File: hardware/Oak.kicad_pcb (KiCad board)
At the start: 2 copper layers, 100 x 40 mm, 73 parts, among them J1 18650 Battery holder, J2 USB_B_Micro, J3 Conn_Coaxial, J4 Conn_ARM_JTAG_SWD_10, SW1 SW_SPDT, SW2 SW_Push, U1 AP2112, U2 ATSAMD21, U3 MCP7383, U4 PA1010D, U5 RFM95, U6 Waveshare_1in54_epaper

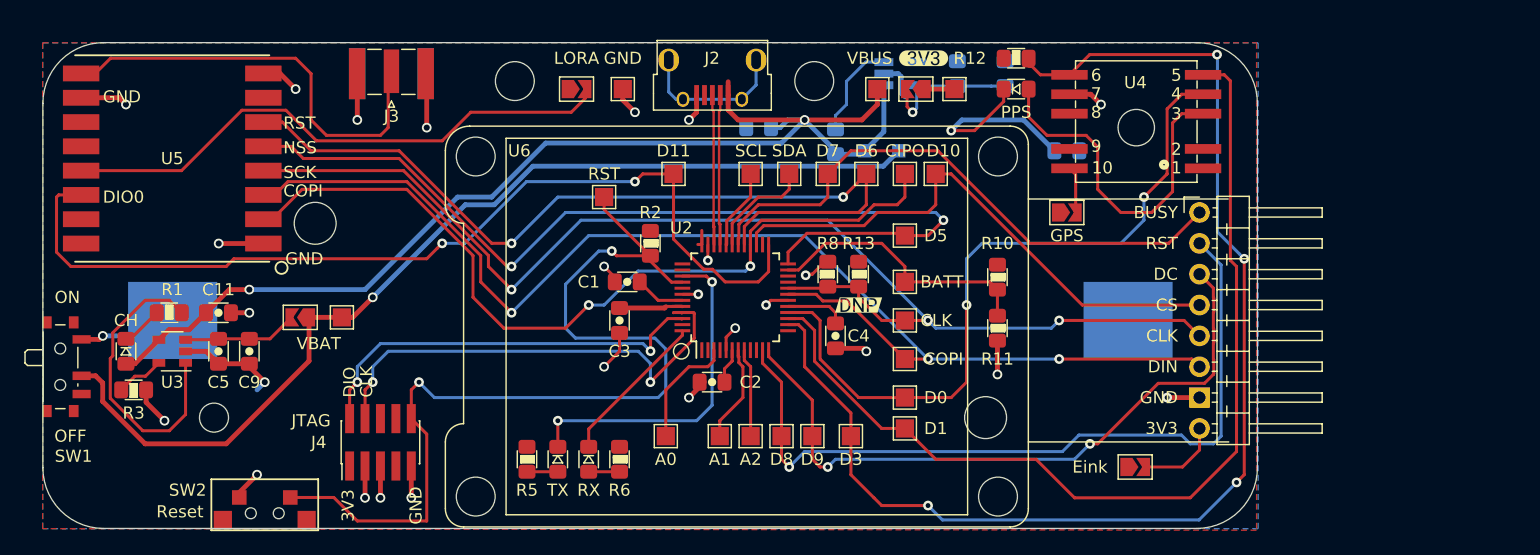
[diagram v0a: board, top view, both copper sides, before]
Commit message: refactor: regenerate drill map files
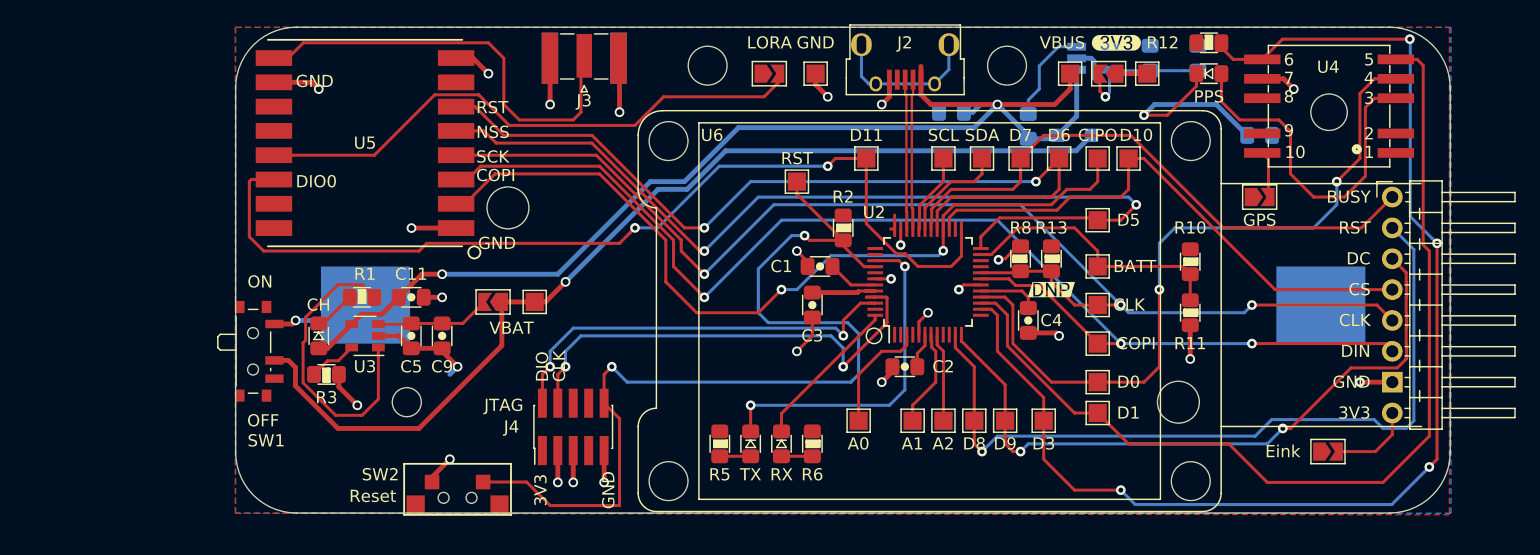
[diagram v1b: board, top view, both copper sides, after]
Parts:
- moved D2 15.9 mm to (45.5, 57.1)
- moved REF** 15.9 mm to (44.5, 66.2)
- moved C1 15.9 mm to (86.7, 51.4)
- moved C10 15.9 mm to (97.5, 38.7)
- moved C11 15.9 mm to (53.1, 54.0)
- moved C2 15.9 mm to (93.7, 59.7)
- moved C3 15.9 mm to (86.1, 54.6)
- moved C4 15.9 mm to (103.9, 55.9)
- moved C5 15.9 mm to (53.1, 57.1)
- moved C6 15.9 mm to (113.9, 34.3)
- moved C7 15.9 mm to (117.8, 34.3)
- moved C9 15.9 mm to (55.6, 57.1)
- moved D1 15.9 mm to (107.7, 40.6)
- moved D3 15.9 mm to (118.7, 35.6)
- moved D4 15.9 mm to (81.0, 66.0)
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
